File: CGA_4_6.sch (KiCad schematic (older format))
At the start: 5 parts, among them U1 74S112, U2 74LS74, U26 74S04, U46 74LS00, U47 74LS51

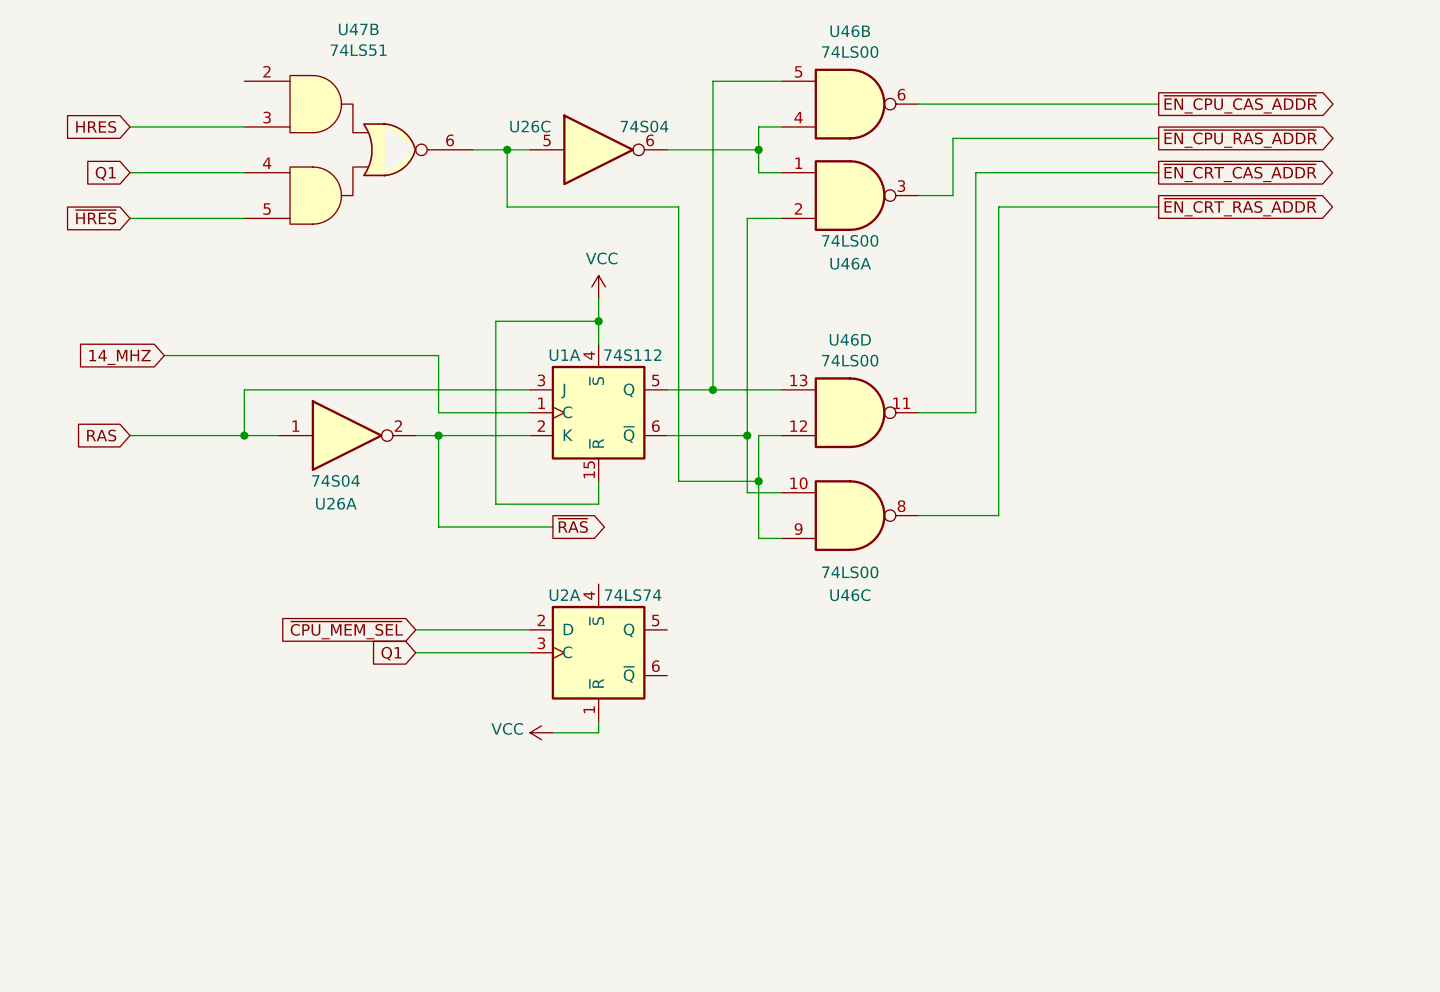
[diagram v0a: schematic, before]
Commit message: More sheet 4
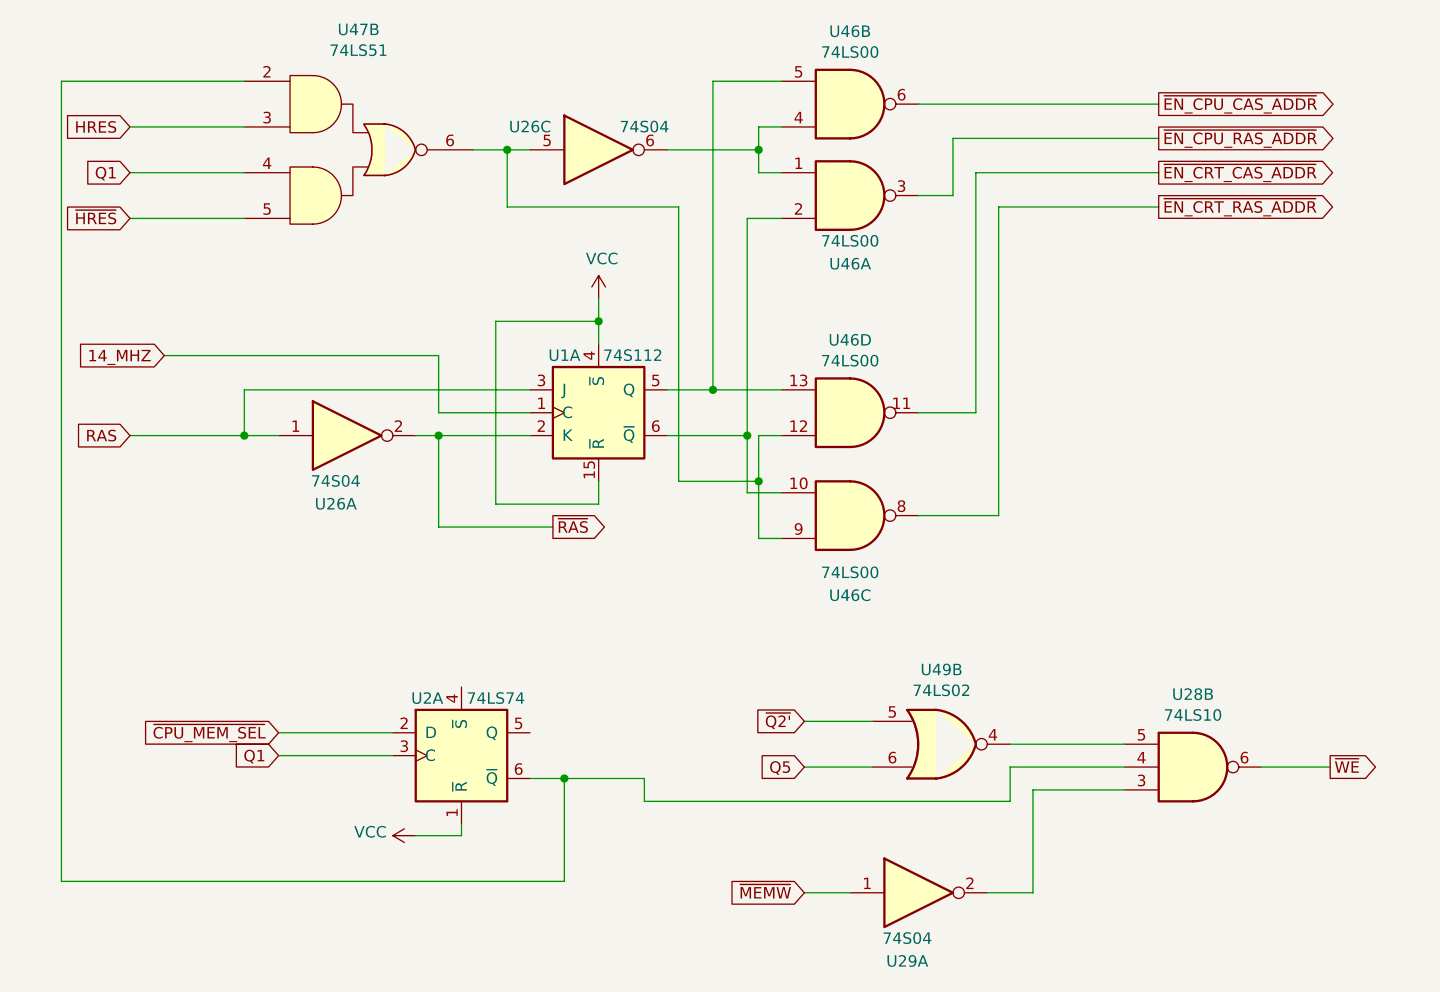
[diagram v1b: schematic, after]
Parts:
- added U28: 74LS10, Package_DIP:DIP-14_W7.62mm_LongPads, symbol 74xx:74LS10
- added U29: 74S04, Package_DIP:DIP-14_W7.62mm_LongPads, symbol 74xx:74LS04
- added U49: 74LS02, Package_DIP:DIP-14_W7.62mm_LongPads, symbol 74xx:74LS02
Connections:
- net at U47.2: now also U2.6 (~Q), U28.4
- new net: U28.5, U49.4
- new net: U28.3, U29.2
- new net Q5: U49.6
- new net ~MEMW: U29.1
- new net ~Q2': U49.5
- new net ~WE: U28.6
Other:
- moved on the sheet: U2A
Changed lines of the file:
@@
 L 74xx:74LS74 U2
 U 1 1 62D7E32E
-P 2900 3400
-F 0 "U2" H 2750 3650 50  0000 C CNN
-F 1 "74LS74" H 3050 3650 50  0000 C CNN
-F 2 "Package_DIP:DIP-14_W7.62mm_LongPads" H 2900 3400 50  0001 C CNN
-F 3 "74xx/74hc_hct74.pdf" H 2900 3400 50  0001 C CNN
-	1    2900 3400
+P 2300 3850
+F 0 "U2" H 2150 4100 50  0000 C CNN
+F 1 "74LS74" H 2450 4100 50  0000 C CNN
+F 2 "Package_DIP:DIP-14_W7.62mm_LongPads" H 2300 3850 50  0001 C CNN
+F 3 "74xx/74hc_hct74.pdf" H 2300 3850 50  0001 C CNN
+	1    2300 3850
 	1    0    0    -1
 $EndComp
-Text GLabel 2100 3300 0    50   Input ~ 0
+Text GLabel 1500 3750 0    50   Input ~ 0
 ~CPU_MEM_SEL
 $Comp
 L power:VCC #PWR?
 U 1 1 62D8D7F8
-P 2700 3750
-F 0 "#PWR?" H 2700 3600 50  0001 C CNN
-F 1 "VCC" V 2715 3877 50  0000 L CNN
-F 2 "" H 2700 3750 50  0001 C CNN
-F 3 "" H 2700 3750 50  0001 C CNN
-	1    2700 3750
+P 2100 4200
+F 0 "#PWR?" H 2100 4050 50  0001 C CNN
+F 1 "VCC" V 2115 4327 50  0000 L CNN
+F 2 "" H 2100 4200 50  0001 C CNN
+F 3 "" H 2100 4200 50  0001 C CNN
+	1    2100 4200
 	0    -1   -1   0
 $EndComp
 Wire Wire Line
-	2700 3750 2900 3750
+	2100 4200 2300 4200
 Wire Wire Line
-	2900 3750 2900 3700
+	2300 4200 2300 4150
 Wire Wire Line
-	2600 3400 2100 3400
-Text GLabel 2100 3400 0    50   Input ~ 0
+	2000 3850 1500 3850
+Text GLabel 1500 3850 0    50   Input ~ 0
 Q1
 Wire Wire Line
-	2100 3300 2600 3300
+	1500 3750 2000 3750
 Wire Wire Line
 	4300 1000 5350 1000
@@
 Text GLabel 2700 2850 2    50   Output ~ 0
 ~RAS
+$Comp
+L 74xx:74LS02 U49
+U 2 1 62E07279
+P 4400 3800
+F 0 "U49" H 4400 4125 50  0000 C CNN
+F 1 "74LS02" H 4400 4034 50  0000 C CNN
+F 2 "Package_DIP:DIP-14_W7.62mm_LongPads" H 4400 3800 50  0001 C CNN
+F 3 "http://www.ti.com/lit/gpn/sn74ls02" H 4400 3800 50  0001 C CNN
+	2    4400 3800
+	1    0    0    -1
+$EndComp
+Text GLabel 3800 3700 0    50   Input ~ 0
+~Q2'
+Wire Wire Line
+	3800 3700 4100 3700
+Text GLabel 3800 3900 0    50   Input ~ 0
+Q5
+Wire Wire Line
+	3800 3900 4100 3900
+$Comp
+L 74xx:74LS10 U28
+U 2 1 62E3583A
+P 5500 3900
+F 0 "U28" H 5500 3583 50  0000 C CNN
+F 1 "74LS10" H 5500 3674 50  0000 C CNN
+F 2 "Package_DIP:DIP-14_W7.62mm_LongPads" H 5500 3900 50  0001 C CNN
+F 3 "http://www.ti.com/lit/gpn/sn74LS10" H 5500 3900 50  0001 C CNN
+	2    5500 3900
+	1    0    0    1
+$EndComp
+Wire Wire Line
+	4700 3800 5200 3800
+Wire Wire Line
+	2600 3950 2750 3950
+Wire Wire Line
+	3100 3950 3100 4050
+Wire Wire Line
+	3100 4050 4700 4050
+Wire Wire Line
+	4700 4050 4700 3900
+Wire Wire Line
+	4700 3900 5200 3900
+Wire Wire Line
+	2750 3950 2750 4400
+Wire Wire Line
+	2750 4400 550  4400
+Wire Wire Line
+	550  4400 550  900
+Wire Wire Line
+	550  900  1350 900
+Connection ~ 2750 3950
+Wire Wire Line
+	2750 3950 3100 3950
+$Comp
+L 74xx:74LS04 U?
+U 1 1 62E66435
+P 4300 4450
+AR Path="/60463C57/62E66435" Ref="U?"  Part="2"
+AR Path="/60463CC5/62E66435" Ref="U29"  Part="1"
+F 0 "U29" H 4250 4150 50  0000 C CNN
+F 1 "74S04" H 4250 4250 50  0000 C CNN
+F 2 "Package_DIP:DIP-14_W7.62mm_LongPads" H 4300 4450 50  0001 C CNN
+F 3 "http://www.ti.com/lit/gpn/sn74LS04" H 4300 4450 50  0001 C CNN
+	1    4300 4450
+	1    0    0    -1
+$EndComp
+Wire Wire Line
+	5200 4000 4800 4000
+Wire Wire Line
+	4800 4000 4800 4450
+Wire Wire Line
+	4800 4450 4600 4450
+Text GLabel 3800 4450 0    50   Input ~ 0
+~MEMW
+Wire Wire Line
+	3800 4450 4000 4450
+Text GLabel 6100 3900 2    50   Output ~ 0
+~WE
+Wire Wire Line
+	5800 3900 6100 3900
 $EndSCHEMATC
